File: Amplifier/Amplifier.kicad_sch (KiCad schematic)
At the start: 44 parts, among them J1 Conn_01x01_Pin, J10 Conn_01x01_Pin, J11 Conn_01x01_Pin, J2 Conn_01x01_Pin, J3 Conn_Shielded_Pair, J4 Conn_Shielded_Pair, J5 Conn_Shielded_Pair, J6 Conn_Shielded_Pair, J9 Conn_01x10, Q1 JFE2140D, Q2 Q_NJFET_DSG, U10 AD40xxBRMZ, U11 LP5907MFX-1.8, U12 ADA4940-1xCP, U16 LTC6268xS8, U2 LMP7721

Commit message: Signed-off-by: lokimetasmith <lokimail@gmail.com>
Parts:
- removed C2: 100nF, Capacitor_SMD:C_0805_2012Metric, symbol Device:C
- removed C3: 100nF, Capacitor_SMD:C_0402_1005Metric, symbol Device:C
- removed C4, C5: 10nF, Capacitor_SMD:C_0402_1005Metric, symbol Device:C
- removed C_BIAS_FILT: 1uF, Capacitor_SMD:C_0402_1005Metric, symbol Device:C
- removed D_WEEP_CLAMP: BAT54, Diode_SMD:D_SOD-323, symbol Diode:BAT54
- removed H1: Nanopore, footprints:Nanopore holder_recessed, symbol Mechanical:MountingHole
- removed J1, J10, J11, J2: Conn_01x01_Pin, footprints:Electrode_Guard_Shield, symbol Connector:Conn_Coaxial_Small
- removed J3, J4, J5, J6: Conn_Shielded_Pair, symbol Connector:Conn_Shielded_Pair
- removed J9: Conn_01x10, Connector_JST:JST_SH_SM10B-SRSS-TB_1x10-1MP_P1.00mm_Horizontal, symbol MR1:Conn_01x11_MP
- removed Q_WEEP: 2N7002, Package_TO_SOT_SMD:SOT-23, symbol Transistor_FET:2N7002
- removed R9: 100, Resistor_SMD:R_0805_2012Metric, symbol Device:R
- removed R_BIAS_FILT: 1k (0.1%), Resistor_SMD:R_0402_1005Metric, symbol Device:R
- removed R_WEEP_GATE: 1M, Resistor_SMD:R_0402_1005Metric, symbol Device:R
- removed R_WEEP_LIM, R_WEEP_PULL: 100k, Resistor_SMD:R_0402_1005Metric, symbol Device:R
- removed U10: AD40xxBRMZ, Package_SO:MSOP-10_3x3mm_P0.5mm, symbol Analog_ADC:AD40xxBRMZ
- removed U11: LP5907MFX-1.8, Package_TO_SOT_SMD:SOT-23-5, symbol Regulator_Linear:LP5907MFX-1.8
- removed U12: ADA4940-1xCP, Package_CSP:LFCSP-16-1EP_3x3mm_P0.5mm_EP1.3x1.3mm_ThermalVias, symbol Amplifier_Difference:ADA4940-1xCP
- added C10, C12, C31, C32, C33, C39: 100nF, Capacitor_SMD:C_0402_1005Metric, symbol Device:C
- added C11: 4.7u, Capacitor_SMD:C_0402_1005Metric, symbol Device:C_Small
- added C29, C30: 10pF, Capacitor_SMD:C_0402_1005Metric, symbol Device:C
- added C35: 10u, Capacitor_SMD:C_0402_1005Metric, symbol Device:C_Small
- added C41: 1nF, Capacitor_SMD:C_0402_1005Metric, symbol Device:C_Small
- added C7, C8: 10nF, Capacitor_SMD:C_0402_1005Metric, symbol Device:C
- added D82: MBR0540, Diode_SMD:D_SOD-123, symbol Diode:MBR0540
- added J7: Conn_01x14_MountingPin, symbol Connector_Generic_MountingPin:Conn_01x14_MountingPin
- added NT7, NT8: NetTie_2, NetTie:NetTie-2_SMD_Pad0.5mm, symbol Device:NetTie_2
- added Q3: 2N7002, Package_TO_SOT_SMD:SOT-23, symbol Transistor_FET:2N7002
- added R14, R15: 100k, symbol Device:R
- added R16: 1M, Resistor_SMD:R_0402_1005Metric, symbol Device:R
- added R27, R41: 27, Resistor_SMD:R_0402_1005Metric, symbol Device:R_Small_US
- added R28, R29, R30, R31: 49.9, Resistor_SMD:R_0402_1005Metric, symbol Device:R_Small_US
- added R43, R44, R45, R46: 499 (0.1%), Resistor_SMD:R_0402_1005Metric, symbol Device:R
- added U13: AD40xxBRMZ, Package_SO:MSOP-10_3x3mm_P0.5mm, symbol Analog_ADC:AD40xxBRMZ
- added U14: LP5907MFX-1.8, Package_TO_SOT_SMD:SOT-23-5, symbol Regulator_Linear:LP5907MFX-1.8
- added U6: ADA4940-1xCP, Package_CSP:LFCSP-16-1EP_3x3mm_P0.5mm_EP1.3x1.3mm_ThermalVias, symbol Amplifier_Difference:ADA4940-1xCP
- J_POGO1: symbol Amplifier:PogoPin_SpringHeader_6Pin_Array -> MR1:PogoPin_SpringHeader_6Pin_Array
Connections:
- net WEEP_SENSE is gone; now on net GNDA: J_POGO1.3 (GNDA)
- net >PORE_AMP: now also J_POGO1.6 (WE_POS), J7.14 (Pin_14); no longer J_POGO1.1 (CE_GNDA)
- net CE_GNDA: now also J_POGO1.1 (CE_GNDA), NT8.1; no longer J_POGO1.6 (WE_POS)
- net GDAC_CLK: now also R31.1, U13.8 (SCK)
- net GNDA: now also C10.2, C12.2, C29.1, C30.2, C31.2, C32.2, C33.2, C35.2, C39.2, C7.2, C8.2, D82.2 (A), J7.11 (Pin_11), J7.13 (Pin_13), J7.9 (Pin_9), NT8.2, Q3.2 (S), R43.1, U13.5 (GND), U6.17 (EP), U6.9 (VOCM); no longer J_POGO1.4 (WEEP_SENSE), NT4.2, NT5.2, Q2.1 (D), Q2.2 (S)
- net RE_TRANS: now also J_POGO1.2 (RE_TRANS), R6.2; no longer J_POGO1.5 (WS_CIS)
- net VDDA: now also C10.1, C31.1, C7.1, J7.10 (Pin_10), U6.5 (+Vs), U6.6 (+Vs), U6.7 (+Vs), U6.8 (+Vs)
- net VSSA: now also C12.1, C32.1, C8.1, J7.12 (Pin_12), U6.13 (-Vs), U6.14 (-Vs), U6.15 (-Vs), U6.16 (-Vs)
- net Vbias: now also C35.1, U13.1 (REF)
- net WS_CIS: now also C1.2, J_POGO1.5 (WS_CIS), R1.2, U2.8 (-); no longer J_POGO1.2 (RE_TRANS)
- net Signal_AMP: now reaches R3.1, U16.6
- net Signal_AMP: now also R45.1
- net Virtual_Ground: now reaches R3.2, R4.2, U16.2 (-)
- new net: C30.1, C41.2, R41.2, U13.4 (IN-)
- new net: J7.7 (Pin_7), R30.2
- new net: R43.2, R44.1, U6.3 (-IN)
- new net: R44.2, U6.4 (+FB)
- new net: C29.2, C41.1, R27.2, U13.3 (IN+)
- new net: C39.1, NT7.1
- new net: Q3.1 (G), R16.2
- new net: R41.1, U6.11 (-OUT)
- new net: J7.3 (Pin_3), R31.2
- new net: J7.5 (Pin_5), R28.2
- new net: J7.6 (Pin_6), R29.2
- new net: R45.2, R46.2, U6.2 (+IN)
- new net: R27.1, U6.10 (+OUT)
- new net: R46.1, U6.1 (-FB)
- new net +1V8: C11.1, U13.2 (VDD), U14.5 (OUT)
- new net +3V3: C33.1, J7.1 (Pin_1), R14.1, U13.10 (VIO), U14.1 (IN)
- new net GDAC_EN: R30.1, U13.6 (CNV)
- new net GDAC_SDI: R29.1, U13.9 (SDI)
- new net GDAC_SDO: R28.1, U13.7 (SDO)
- new net GND: C11.2, J7.2 (Pin_2), J7.4 (Pin_4), J7.8 (Pin_8), U14.2 (GND)
- new net R_WEEP_GATE: D82.1 (K), R15.2, R16.1
- new net R_WEEP_LIM: J_POGO1.4 (WEEP_SENSE), R15.1
- new net R_WEEP_PULL: Q3.3 (D), R14.2, U14.3 (EN)
- new net SHIELD: NT7.2
- new net SHIELD_AMP: J7.MP (MountPin), NT4.2
- new net Vbias_AMP: NT5.2, Q2.1 (D), Q2.2 (S)
- no-connect marks 0 -> 2
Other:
- note added: "RF-damping capacitor"
- note added: "R_DAMP"
- note added: "Stage 1: Transimpedance Amp"
- note added: "we need to play back a waveform"
- moved on the sheet: C1, C19, C20, C6, J_POGO1, NT3, NT4, NT5, Q1A, Q1B, Q1C, Q2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

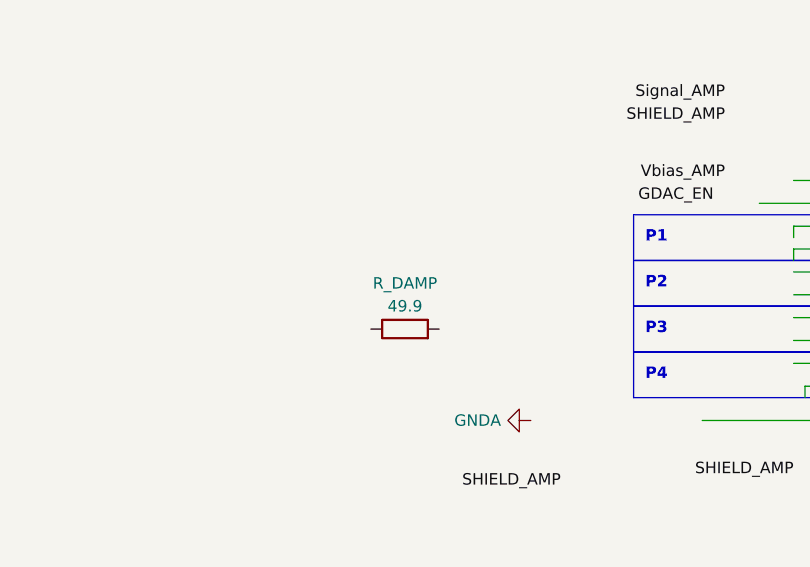
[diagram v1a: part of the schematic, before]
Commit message: updated amplifier
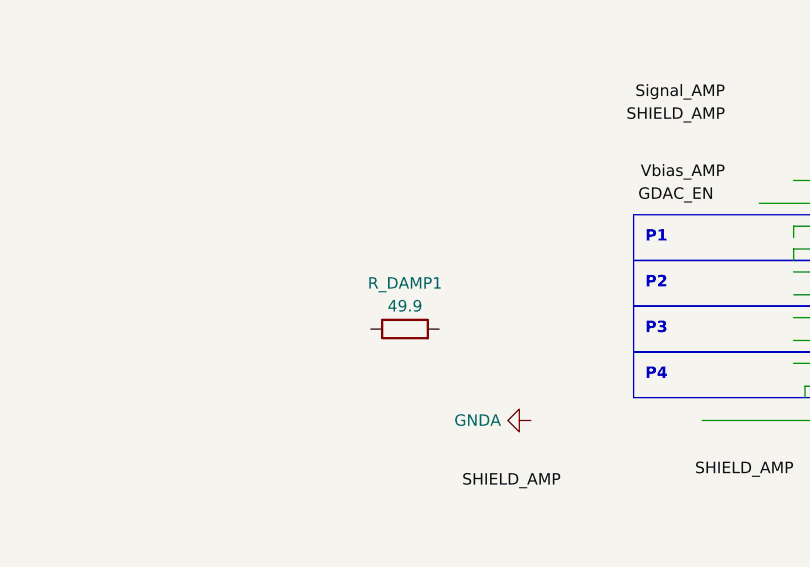
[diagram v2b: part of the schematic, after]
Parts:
- R14, R15: footprint (none) -> Resistor_SMD:R_0402_1005Metric
- renumbered R_DAMP to R_DAMP1
